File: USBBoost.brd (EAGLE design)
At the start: 43.8 x 20.3 mm, 27 parts, among them IC1 RT9276, J1 Input, J2 3.75V, J3 2.33V, J4 1.17V, J5 Status, X1 USB_

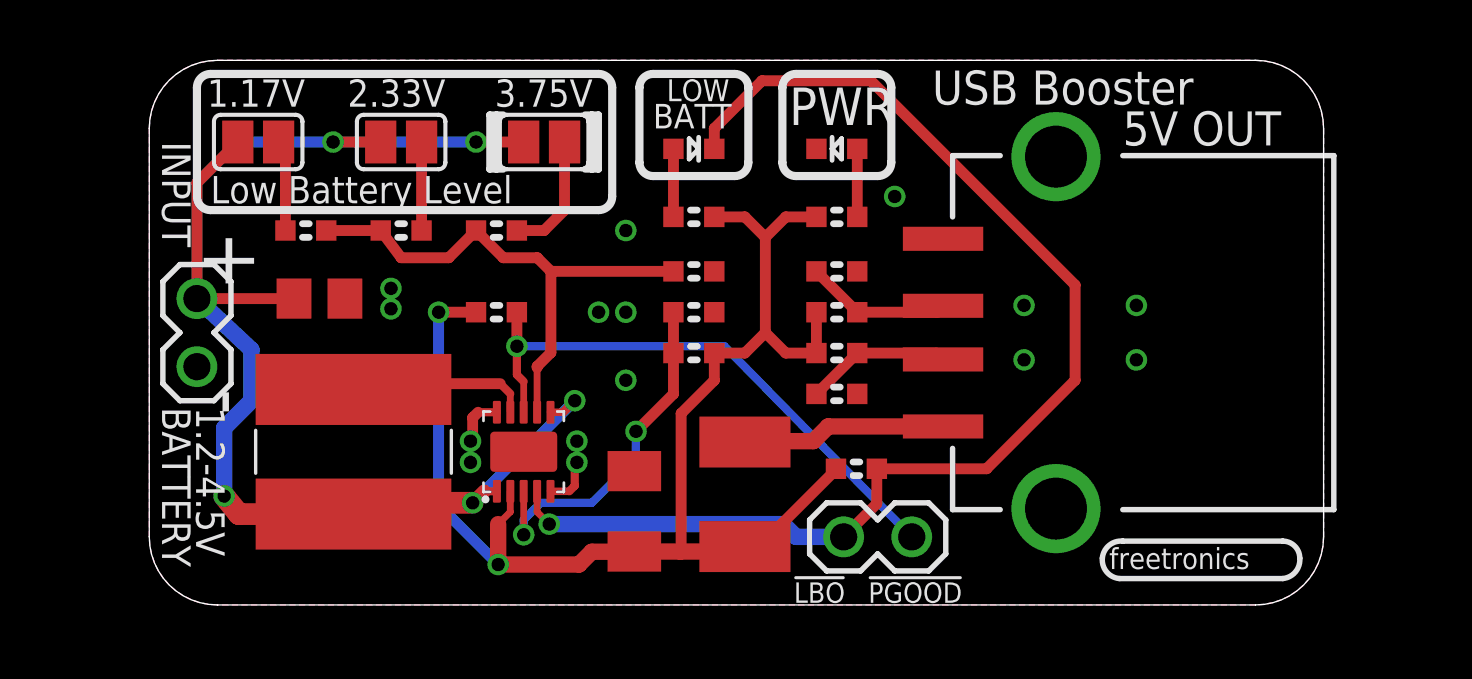
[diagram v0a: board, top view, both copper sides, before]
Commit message: Overlay improvements
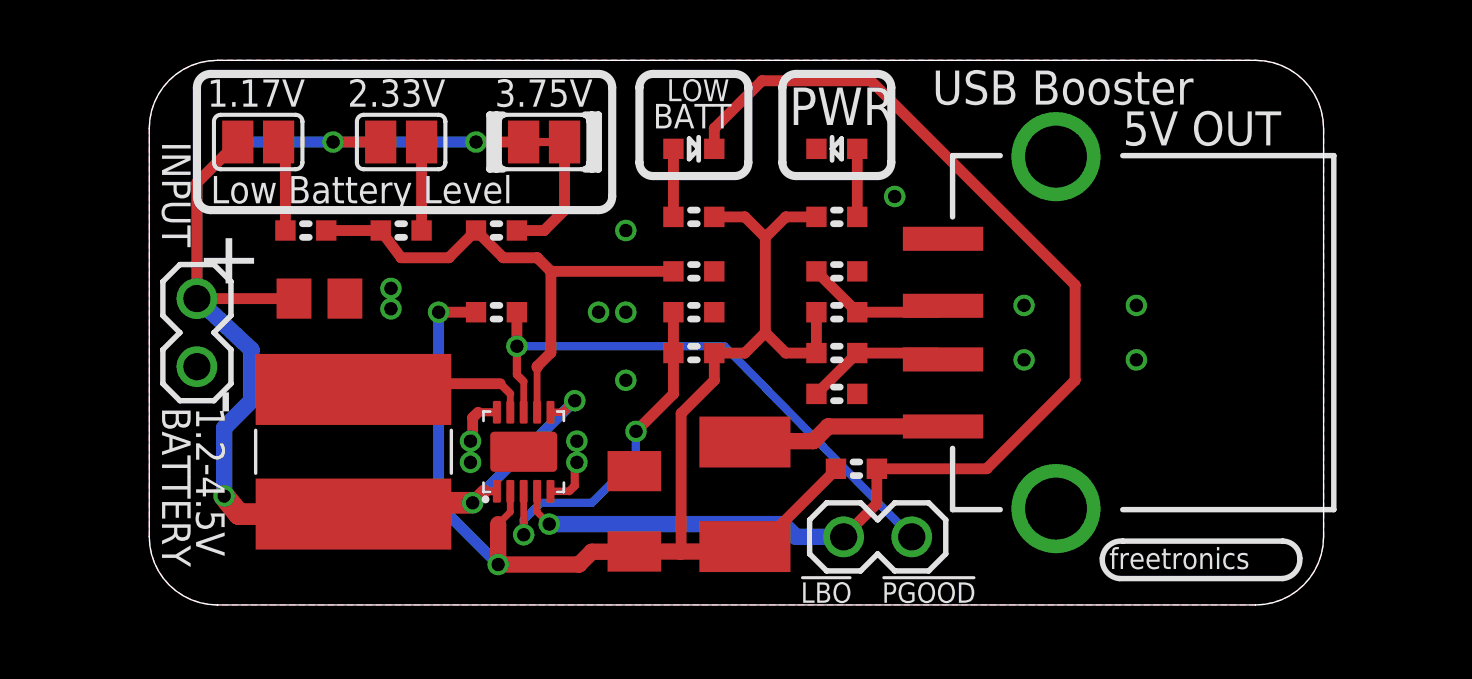
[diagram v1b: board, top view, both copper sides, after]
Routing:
- net N$1: track 0.00 -> 1.02 mm
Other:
- board text added: "LBO: Low Battery Output"
- board text added: "PGOOD: Power Good"
- board text added: "www.freetronics.com"
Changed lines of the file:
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@@
 <grid distance="0.01" unitdist="inch" unit="inch" style="lines" multiple="1" display="yes" altdistance="3.125" altunitdist="mil" altunit="mil"/>
 <layers>
-<layer number="1" name="Top" color="4" fill="1" visible="no" active="yes"/>
+<layer number="1" name="Top" color="4" fill="1" visible="yes" active="yes"/>
 <layer number="2" name="Route2" color="1" fill="3" visible="no" active="no"/>
 <layer number="3" name="Route3" color="4" fill="3" visible="no" active="no"/>
@@
 <layer number="14" name="Route14" color="1" fill="6" visible="no" active="no"/>
 <layer number="15" name="Route15" color="4" fill="6" visible="no" active="no"/>
-<layer number="16" name="Bottom" color="1" fill="1" visible="no" active="yes"/>
+<layer number="16" name="Bottom" color="1" fill="1" visible="yes" active="yes"/>
 <layer number="17" name="Pads" color="2" fill="1" visible="yes" active="yes"/>
 <layer number="18" name="Vias" color="2" fill="1" visible="yes" active="yes"/>
 <layer number="19" name="Unrouted" color="14" fill="1" visible="yes" active="yes"/>
 <layer number="20" name="Dimension" color="15" fill="1" visible="yes" active="yes"/>
-<layer number="21" name="tPlace" color="16" fill="1" visible="no" active="yes"/>
+<layer number="21" name="tPlace" color="16" fill="1" visible="yes" active="yes"/>
 <layer number="22" name="bPlace" color="14" fill="1" visible="yes" active="yes"/>
 <layer number="23" name="tOrigins" color="15" fill="1" visible="yes" active="yes"/>
@@
 <wire x1="42.291" y1="2.3813" x2="42.926" y2="1.7463" width="0.2032" layer="21" curve="-90.036103"/>
 <wire x1="42.926" y1="1.7463" x2="42.291" y2="0.9843" width="0.2032" layer="21" curve="-89.969931"/>
-<wire x1="38.481" y1="9.6679" x2="38.481" y2="3.5719" width="0.2032" layer="22"/>
-<wire x1="38.481" y1="3.5719" x2="39.243" y2="2.9369" width="0.2032" layer="22" curve="90.075241"/>
-<wire x1="39.243" y1="2.9369" x2="39.878" y2="3.6989" width="0.2032" layer="22" curve="90.030084"/>
-<wire x1="39.878" y1="3.6989" x2="39.878" y2="9.6679" width="0.2032" layer="22"/>
-<wire x1="39.878" y1="9.6679" x2="39.243" y2="10.3029" width="0.2032" layer="22" curve="90.036103"/>
-<wire x1="39.243" y1="10.3029" x2="38.481" y2="9.6679" width="0.2032" layer="22" curve="89.969931"/>
 <text x="2.032" y="13.97" size="2.1844" layer="21" font="vector" ratio="20" rot="SR270">+</text>
 <text x="23.876" y="17.907" size="1.397" layer="21" font="vector" ratio="15">PWR</text>
@@
 <text x="35.814" y="1.3399" size="0.7874" layer="21" font="vector" ratio="18">freetronics</text>
 <text x="29.21" y="18.669" size="1.27" layer="21" font="vector" ratio="15">USB Booster</text>
-<text x="30.988" y="13.716" size="1.016" layer="22" font="vector" ratio="15" rot="MR0">SKU:USBBOOST</text>
-<text x="38.8366" y="3.1909" size="0.7874" layer="22" font="vector" ratio="18" rot="MR90">freetronics</text>
-<text x="30.988" y="15.748" size="1.016" layer="22" font="vector" ratio="15" rot="MR0">www.freetronics.com/usbboost</text>
+<text x="12.446" y="18.034" size="1.016" layer="22" font="vector" ratio="15" rot="MR0">SKU:USBBOOST</text>
+<text x="29.972" y="16.002" size="1.016" layer="22" font="vector" ratio="15" rot="MR0">www.freetronics.com/usbboost</text>
 <text x="2.54" y="14.224" size="1.397" layer="22" font="vector" ratio="20" rot="SMR270">+</text>
 <text x="2.54" y="7.3025" size="1.397" layer="22" font="vector" ratio="20" rot="SMR270">-</text>
-<text x="30.861" y="17.272" size="1.4224" layer="22" font="vector" ratio="15" rot="MR0">USB Booster</text>
+<text x="31.242" y="18.034" size="1.4224" layer="22" font="vector" ratio="15" rot="MR0">USB Booster</text>
 <text x="19.304" y="18.796" size="0.8128" layer="21" font="vector" ratio="15">LOW</text>
 <text x="2.159" y="18.589625" size="1.016" layer="21" font="vector" ratio="15">1.17V</text>
@@
 <text x="12.8905" y="18.589625" size="1.016" layer="21" font="vector" ratio="15">3.75V</text>
 <text x="1.74625" y="7.381875" size="1.0668" layer="21" font="vector" ratio="16" rot="SR270">1.2-4.5V</text>
-<text x="36.068" y="11.684" size="1.016" layer="22" font="vector" ratio="15" rot="SMR0">Input voltage: 1.2V-4.5V</text>
-<text x="36.068" y="8.89" size="1.016" layer="22" font="vector" ratio="15" rot="SMR0">eg. 2 NiMH or alkaline cells</text>
-<text x="36.068" y="10.16" size="1.016" layer="22" font="vector" ratio="15" rot="SMR0">2.4V min. required for 500mA output.</text>
-<text x="36.068" y="7.366" size="1.016" layer="22" font="vector" ratio="15" rot="SMR0">or lithium ion cell.</text>
+<text x="34.798" y="13.462" size="1.016" layer="22" font="vector" ratio="15" rot="SMR0">Input voltage: 1.2V-4.5V</text>
+<text x="34.798" y="10.414" size="1.016" layer="22" font="vector" ratio="15" rot="SMR0">eg. 2 NiMH or alkaline cells</text>
+<text x="34.798" y="11.938" size="1.016" layer="22" font="vector" ratio="15" rot="SMR0">2.4V min. required for 500mA output.</text>
+<text x="34.798" y="8.89" size="1.016" layer="22" font="vector" ratio="15" rot="SMR0">or lithium ion cell.</text>
 <text x="2.286" y="14.986" size="1.016" layer="21" font="vector" ratio="18">Low Battery Level</text>
-<text x="24.050625" y="0.079375" size="0.762" layer="21" font="vector" ratio="15">!LBO</text>
-<text x="26.82875" y="0.079375" size="0.762" layer="21" font="vector" ratio="15">!PGOOD</text>
+<text x="24.304625" y="0.079375" size="0.762" layer="21" font="vector" ratio="15">!LBO</text>
+<text x="27.33675" y="0.079375" size="0.762" layer="21" font="vector" ratio="15">!PGOOD</text>
 <text x="18.796" y="17.78" size="0.9144" layer="21" font="vector" ratio="15">BATT</text>
 <wire x1="18.796" y1="16.002" x2="21.844" y2="16.002" width="0.3048" layer="21"/>
@@
 <text x="36.322" y="17.145" size="1.27" layer="21" font="vector" ratio="15">5V OUT</text>
 <text x="0.47625" y="17.287875" size="1.0668" layer="21" font="vector" ratio="16" rot="SR270">INPUT</text>
-<text x="30.988" y="3.8735" size="1.016" layer="22" font="vector" ratio="15" rot="MR0">(C)2012 Freetronics Pty Ltd</text>
-<text x="16.51" y="17.272" size="1.016" layer="22" font="vector" ratio="15" rot="MR0">v1.0</text>
+<text x="30.988" y="4.1275" size="1.016" layer="22" font="vector" ratio="15" rot="MR0">(C)2012 Freetronics Pty Ltd</text>
+<text x="16.764" y="18.034" size="1.016" layer="22" font="vector" ratio="15" rot="MR0">v1.0</text>
+<text x="34.798" y="7.112" size="1.016" layer="22" font="vector" ratio="15" rot="SMR0">LBO: Low Battery Output</text>
+<text x="34.798" y="5.842" size="1.016" layer="22" font="vector" ratio="15" rot="SMR0">PGOOD: Power Good</text>
+<text x="30.82925" y="0.079375" size="0.762" layer="22" font="vector" ratio="15" rot="MR0">!PGOOD</text>
+<text x="26.495375" y="0.079375" size="0.762" layer="22" font="vector" ratio="15" rot="MR0">!LBO</text>
+<wire x1="42.545" y1="2.667" x2="42.545" y2="17.272" width="0.4064" layer="22"/>
+<wire x1="38.735" y1="17.272" x2="38.735" y2="2.413" width="0.4064" layer="22"/>
+<wire x1="38.735" y1="2.413" x2="40.259" y2="0.889" width="0.4064" layer="22" curve="89.977447"/>
+<wire x1="40.259" y1="0.889" x2="41.021" y2="0.889" width="0.4064" layer="22"/>
+<wire x1="41.021" y1="0.889" x2="42.545" y2="2.667" width="0.4064" layer="22" curve="90.012891"/>
+<wire x1="42.545" y1="17.272" x2="41.021" y2="19.05" width="0.4064" layer="22" curve="89.993555"/>
+<wire x1="41.021" y1="19.05" x2="40.259" y2="19.05" width="0.4064" layer="22"/>
+<wire x1="40.259" y1="19.05" x2="38.735" y2="17.272" width="0.4064" layer="22" curve="90.012891"/>
+<text x="37.338" y="2.4638" size="1.016" layer="22" font="vector" ratio="15" rot="MR90">www.freetronics.com</text>
+<text x="39.751" y="1.5748" size="1.9304" layer="22" font="vector" ratio="17" rot="MR90">freetronics</text>
 </plain>
 <attributes>
@@
 <wire x1="14.47" y1="8.89775" x2="14.986" y2="9.41375" width="0.4064" layer="1"/>
 </signal>
+<signal name="N$1">
+<wire x1="14.224" y1="17.272" x2="15.24" y2="17.272" width="0.3048" layer="1"/>
+</signal>
 </signals>
+<errors>
+</errors>
 </board>
 </drawing>

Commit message: Final tweaks and DRC for production
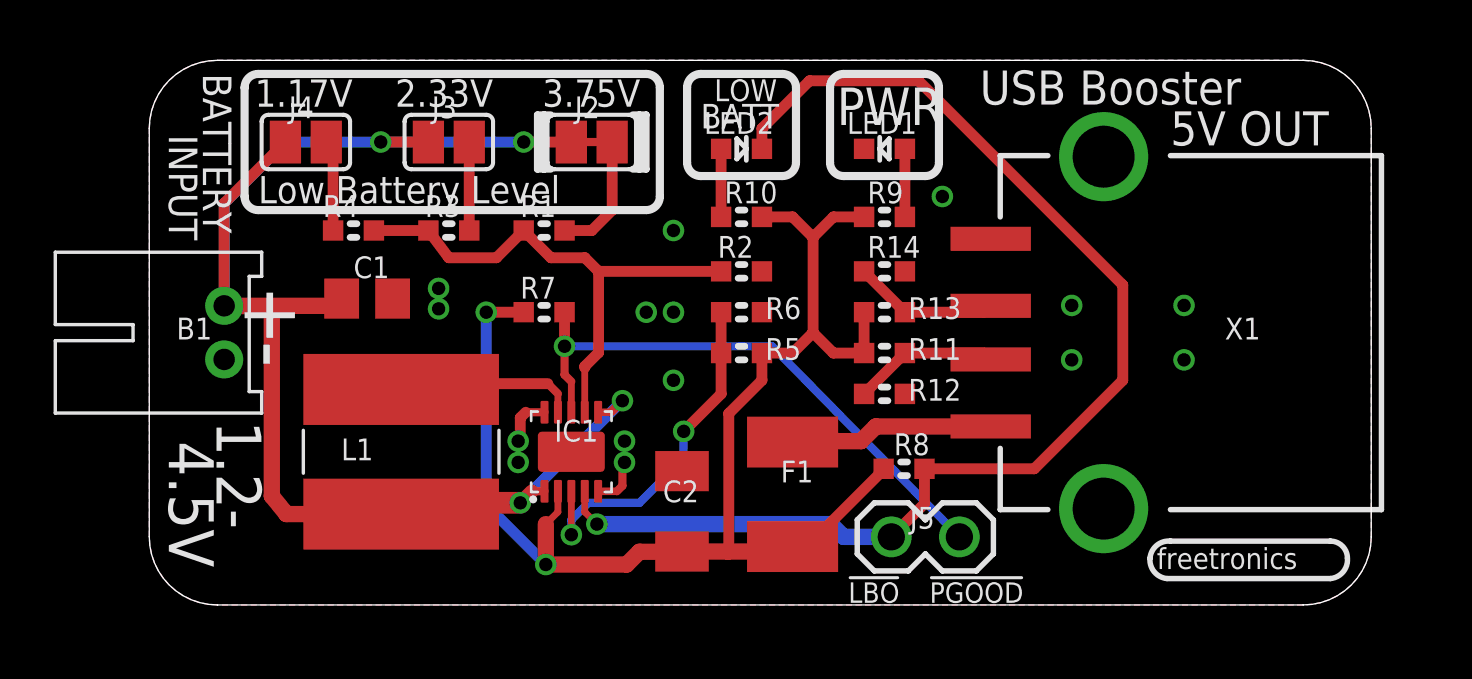
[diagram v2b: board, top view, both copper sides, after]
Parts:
- removed J1: Input, freetronics-master-v1:1X02
- added B1: 2P-JST-PTH, freetronics-jon:FREETRONICS-LUKE_JST-2MM-TH-RA
- C1: value 10uF -> 10uF ceramic
- L1: value 6.8 uH -> 7.4uH
- R1: value 75k -> 130K; device freetronics-original:0603 -> freetronics-master-v1.1:0603
- R10: value 130k -> 1K
- R11: value 73k2 -> 75K
- R12: value 26k7 -> 49K9
- R13: value 20k -> 75K
- R14: value 20k0 -> 49K9
- R2: value 75k -> 20K
- R3: value 49k9 -> 73K2
- R4: value 49k9 -> 26K7
- R5: value 180k -> 180K
- R6: value 10k -> 20K0
- R7: value 10k -> 10K
- R8: value 1k -> 10K
- R9: value 1k -> 2K2
- moved R12 22.4 mm to (27.4, 7.87), turned to 0 degrees
- moved R11 18.6 mm to (27.4, 9.40)
- moved R4 18.1 mm to (7.62, 14.0), turned to 180 degrees
- moved R3 15.7 mm to (11.2, 14.0)
- moved R7 13.0 mm to (14.7, 10.9)
- moved R1 11.8 mm to (14.7, 14.0)
- moved R8 9.73 mm to (28.2, 5.08)
- moved R10 9.16 mm to (22.1, 14.5), turned to 180 degrees
- moved R6 9.14 mm to (22.1, 10.9), turned to 180 degrees
- moved R13 7.27 mm to (27.4, 10.9), turned to 0 degrees
- moved R14 7.27 mm to (27.4, 12.4), turned to 0 degrees
- moved R9 7.11 mm to (27.4, 14.5), turned to 0 degrees
- moved R2 3.87 mm to (22.1, 12.4), turned to 180 degrees
- moved J2 1.78 mm to (16.5, 17.3)
- moved C1 1.78 mm to (8.13, 11.4)
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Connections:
- net !LBO: now also R8.2; no longer R7.2
- net !PGOOD: now also R7.2; no longer R6.2
- net FB: now also R6.2; no longer R14.2
- net GND: now also B1.NEG, R12.2, R14.2, R2.1, R6.1; no longer J1.2, R13.1, R14.1, R3.2, R4.2
- net LBI: now also R1.1, R2.2, R3.1, R4.1; no longer R10.1, R11.1, R12.1, R13.2
- net N$10: now also R13.2, R14.1; no longer R2.2, R4.1
- net N$11: now also R3.2; no longer R11.2
- net N$12: now also R4.2; no longer R12.2
- net N$15: now also R10.2; no longer R9.2
- net N$5: now also R1.2; no longer R10.2
- net N$7: now also R11.2, R12.1; no longer R1.2, R3.1
- net N$8: now also R9.2; no longer R8.2
- net VBAT: now also B1.POS; no longer J1.1
- net VOUT: now also R10.1, R11.1, R13.1; no longer R1.1, R2.1, R6.1
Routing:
- net VBAT: track 55.3 -> 56.7 mm, vias 5 -> 4
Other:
- board size 43.8 x 20.3 mm -> 45.6 x 20.3 mm
- board text added: "1.2-"
- board text added: "4.5V"
- board text removed: "1.2-4.5V"

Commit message: v1.1 release
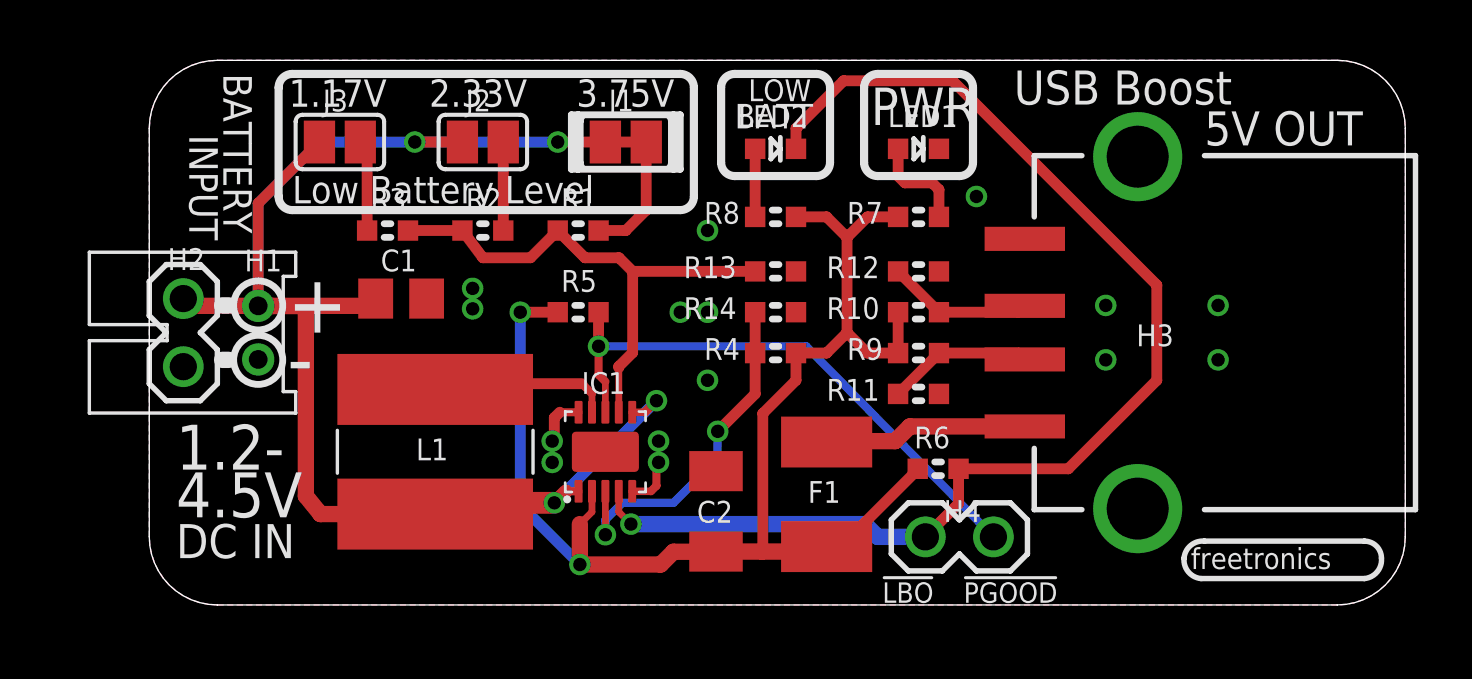
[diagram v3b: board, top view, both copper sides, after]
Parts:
- removed B1: 2P-JST-PTH, freetronics-jon:FREETRONICS-LUKE_JST-2MM-TH-RA
- removed J4: 1.17V, freetronics-luke:SJ
- removed J5: Status, freetronics-master-v1:1X02
- removed X1: USB_, freetronics-master-v1:USB-A-S-SILK-FEMALE
- added H1: 2P-JST-PTH, freetronics-jon:JST-2MM-TH-RA
- added H2: (no value), freetronics-master-v1.1:1X02
- added H3: USB, freetronics-master-v1:USB-A-S-SILK-FEMALE
- added H4: Status, freetronics-master-v1:1X02
- added J1: 3.75V, freetronics-jon:SJC
- C1: value 10uF ceramic -> 10uF ceramic 10V 0805
- C2: value 22uF -> 22uF 10V Ceramic 1206
- F1: value 500mA PTC -> 500mA PTC 1812
- J2: value 3.75V -> 2.33V
- J3: value 2.33V -> 1.17V
- L1: value 7.4uH -> 7.4uH CDRH
- LED1: value Power -> BLUE 0603
- LED2: value Low Batt -> RED 0603
- R1: value 130K -> 130K 0603
- R10: value 1K -> 75K 0603
- R11: value 75K -> 49K9 0603
- R12: value 49K9 -> 49K9 0603
- R13: value 75K -> 20K 0603
- R14: value 49K9 -> 20K0 1% 0603
- R2: value 20K -> 73K2 0603
- R3: value 73K2 -> 26K7 0603
- R4: value 26K7 -> 180K 1% 0603
- R5: value 180K -> 10K 0603
- R6: value 20K0 -> 10K 0603
- R7: value 10K -> 2K2 0603
- R8: value 10K -> 1K 0603
- R9: value 2K2 -> 75K 0603
- moved R4 16.4 mm to (23.4, 9.40)
- moved R7 14.4 mm to (28.7, 14.5)
- moved R8 10.6 mm to (23.4, 14.5), turned to 180 degrees
- moved R2 9.77 mm to (12.4, 14.0), turned to 0 degrees
- moved R6 9.38 mm to (29.4, 5.08), turned to 0 degrees
- moved R10 7.50 mm to (28.7, 10.9), turned to 0 degrees
- moved R5 6.28 mm to (16.0, 10.9), turned to 0 degrees
- moved R9 5.24 mm to (28.7, 9.40)
- moved R12 4.75 mm to (28.7, 12.4)
- moved R13 4.34 mm to (23.4, 12.4), turned to 180 degrees
- moved R14 4.34 mm to (23.4, 10.9), turned to 180 degrees
- moved J2 4.06 mm to (12.4, 17.3)
- moved J3 4.06 mm to (7.11, 17.3)
- moved R3 2.29 mm to (8.89, 14.0), turned to 180 degrees
- moved R11 1.98 mm to (28.7, 7.87)
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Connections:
- removed net N$12 (its old number): J4.1, R4.2
- new net N$11: J2.1, R2.2
- net !LBO: now also H4.2, R6.2; no longer J5.2, R8.2
- net !PGOOD: now also H4.1, R5.2; no longer J5.1, R7.2
- net FB: now also R14.2, R4.2; no longer R5.2, R6.2
- net GND: now also H1.NEG, H2.1, H3.GND, R11.2, R13.1, R14.1; no longer B1.NEG, R14.2, R2.1, R6.1, X1.GND
- net LBI: now also R13.2, R2.1; no longer R2.2, R4.1
- net N$10: now also H3.D+, R10.2, R12.1; no longer R13.2, R14.1, X1.D+
- net N$15: now also R8.2; no longer R10.2
- net N$5: now also J1.1; no longer J2.1
- net N$7: now also H3.D-, R11.1, R9.2; no longer R11.2, R12.1, X1.D-
- net N$8: now also R7.2; no longer R9.2
- net N$9: now also H3.VBUS; no longer X1.VBUS
- net VBAT: now also H1.POS, H2.2, J1.2; no longer B1.POS, J4.2
- net VOUT: now also R4.1, R6.1; no longer R11.1, R13.1
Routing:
- net N$12 (its old number): track 3.41 -> 0.00 mm
- net N$11: track 0.00 -> 3.30 mm
- net VBAT: track 56.7 -> 59.7 mm
- net N$8: track 2.54 -> 3.77 mm
- net N$1: track 1.02 -> 0.00 mm
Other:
- board size 45.6 x 20.3 mm -> 46.9 x 20.3 mm
- board text added: "(C)2013 Freetronics Pty Ltd"
- board text added: "A"
- board text added: "DC IN"
- board text added: "K"
- board text added: "PGOOD: Power Good Output"
- board text added: "USB Boost"
- board text added: "v1.1"
- board text removed: "(C)2012 Freetronics Pty Ltd"
- board text removed: "PGOOD: Power Good"
- board text removed: "USB Booster"
- board text removed: "v1.0"
